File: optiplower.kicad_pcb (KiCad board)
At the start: 2 copper layers, 76.1 x 19 mm, 21 parts, among them J1 Conn_01x02, J2 Conn_01x03, U1 LR7533-M, U2 XL4015, U3 DS2502, U4 ATtiny25-20SS, U5 ATtiny85-20P

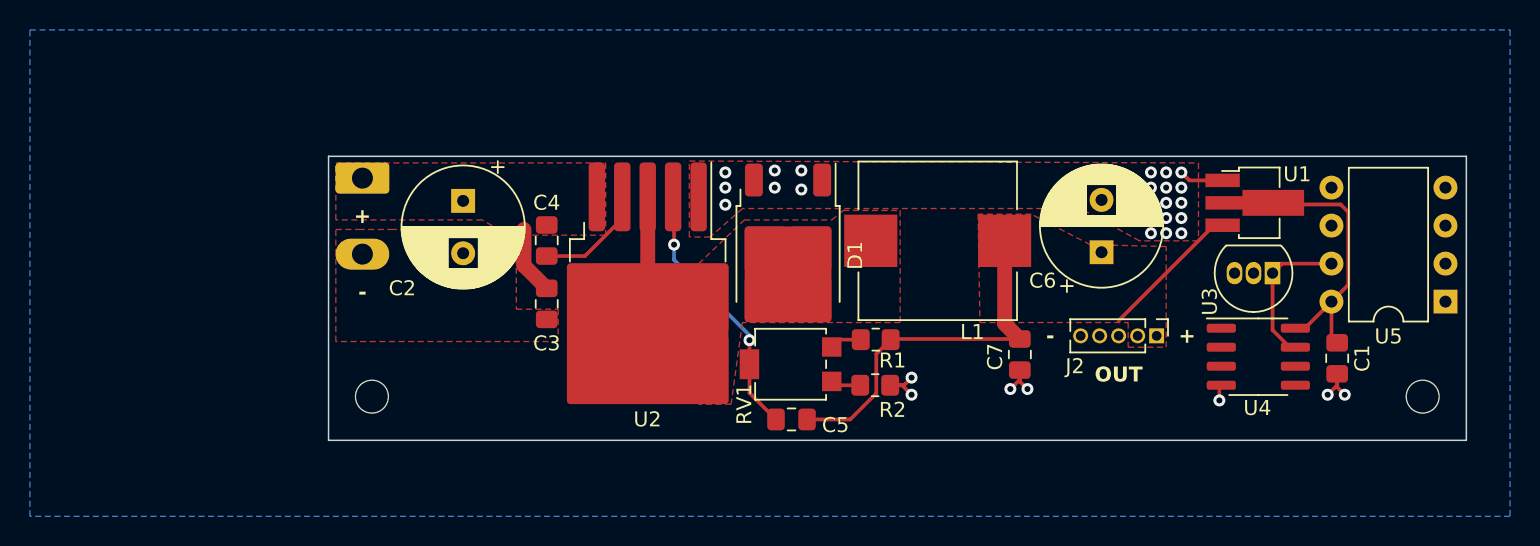
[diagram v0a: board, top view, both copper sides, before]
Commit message: Stuff
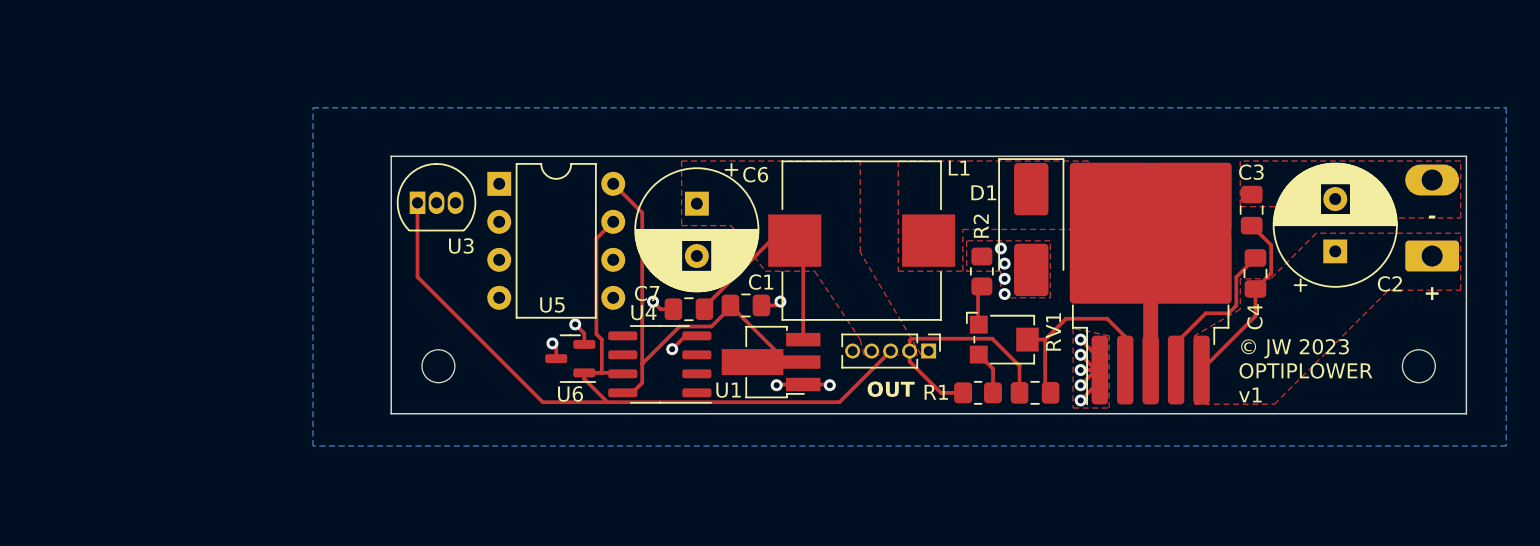
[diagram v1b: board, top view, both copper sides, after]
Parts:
- added U6: DS2502S+, Package_TO_SOT_SMD:SOT-23, F.Cu at (197.0, 91.9)
- D1: value MBRD1045 -> SK84B; footprint Optiplower:TO-252-2 -> Diode_SMD:D_SMB_Handsoldering
- R1: value 15K -> 150K
- R2: value 1K -> 10K
- RV1: value 2K -> 1K; footprint Potentiometer_SMD:Potentiometer_Bourns_3314G_Vertical -> Potentiometer_SMD:Potentiometer_Bourns_TC33X_Vertical
- moved J1 71.7 mm to (254.6, 85.1), turned to 90 degrees
- moved U5 63.7 mm to (192.3, 80.3), turned to 0 degrees
- moved C2 58.4 mm to (248.2, 84.8), turned to 90 degrees
- moved U3 57.3 mm to (186.8, 81.5), turned to 0 degrees
- moved C3 47.5 mm to (242.6, 82.0), turned to 90 degrees
- moved C4 47.4 mm to (242.8, 86.3), turned to 90 degrees
- moved U4 40.0 mm to (203.0, 92.3), turned to 180 degrees
- moved C1 39.7 mm to (208.8, 88.4), turned to 0 degrees
- moved U1 34.6 mm to (210.1, 92.2), turned to 180 degrees
- moved U2 33.8 mm to (235.8, 85.1), turned to 90 degrees
- moved C6 27.2 mm to (205.5, 81.6), turned to -90 degrees
- moved C7 22.3 mm to (205.0, 88.6), turned to 180 degrees
- moved C5 16.4 mm to (228.1, 94.2), turned to 0 degrees
- moved D1 16.3 mm to (227.8, 83.3)
- moved J2 15.3 mm to (221.0, 91.4)
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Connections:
- J2 pad 1: VCC -> GND
- J2 pad 4: GND -> VCC
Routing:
- net /SENSE: track 10.0 -> 57.4 mm
- net +3V3: track 21.1 -> 29.6 mm
- net +24V: track 4.57 -> 12.1 mm
- net GND: track 13.7 -> 20.8 mm, vias 29 -> 16
- net Net-(U2-FB): track 17.7 -> 13.5 mm, vias 2 -> 0
- net VCC: track 34.6 -> 30.7 mm
- net Net-(U2-VC): track 7.55 -> 10.6 mm
- net Net-(R1-Pad2): track 2.14 -> 2.95 mm
- net Net-(R2-Pad1): track 2.01 -> 2.58 mm
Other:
- board size 76.1 x 19 mm -> 71.9 x 17.2 mm
- board text added: "© JW 2023 OPTIPLOWER v1"
